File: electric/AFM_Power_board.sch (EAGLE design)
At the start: 16 parts, among them IC1 LM4041CILP, IC2 LM7805_TO220V, IC3 7812T, J2 694103303002

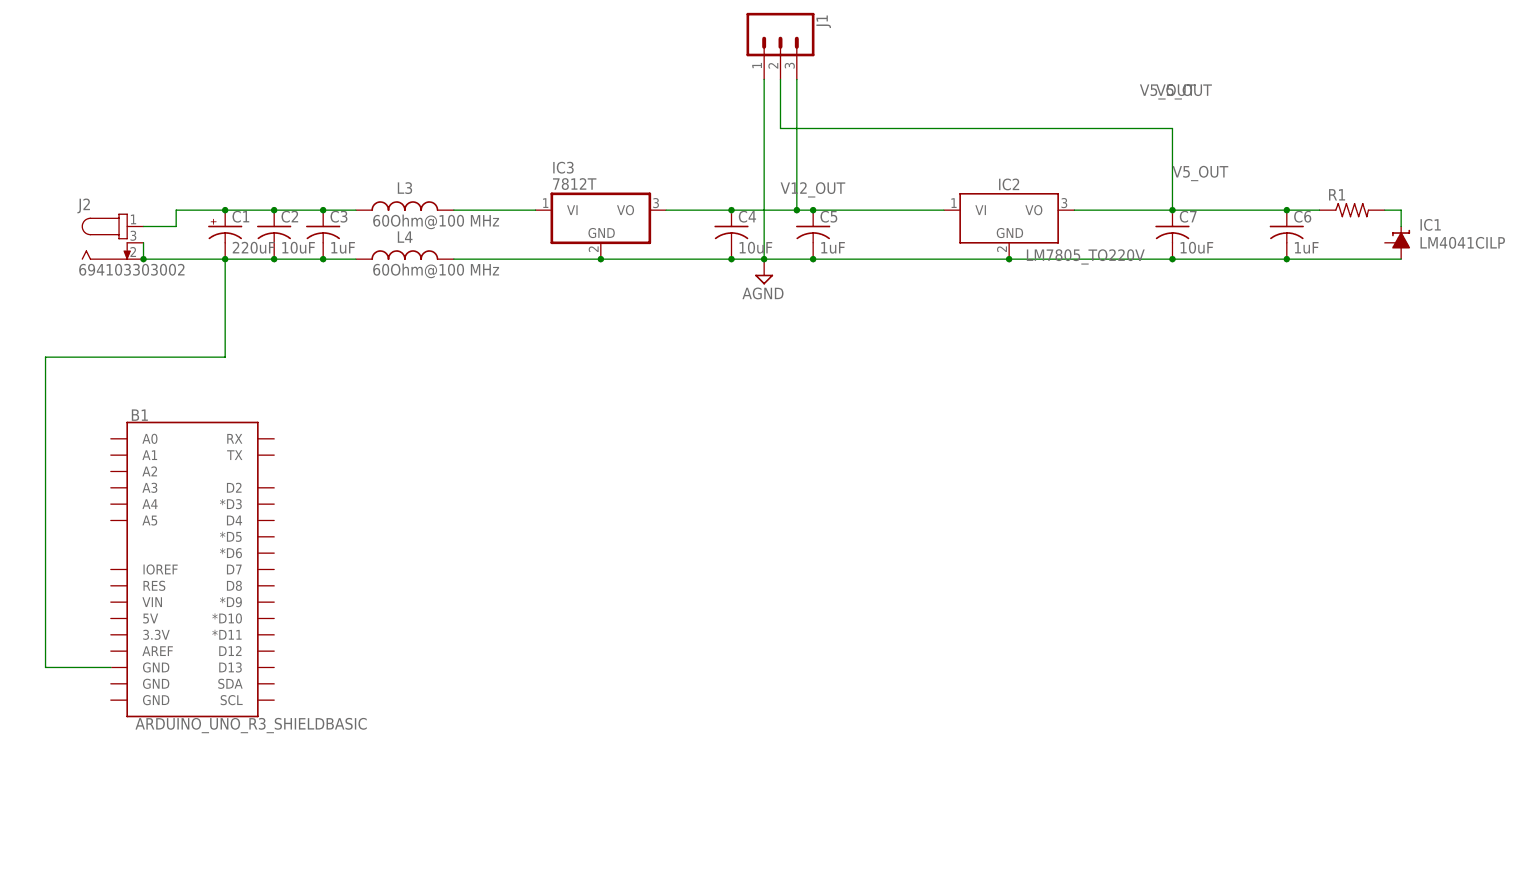
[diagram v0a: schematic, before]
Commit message: allboards
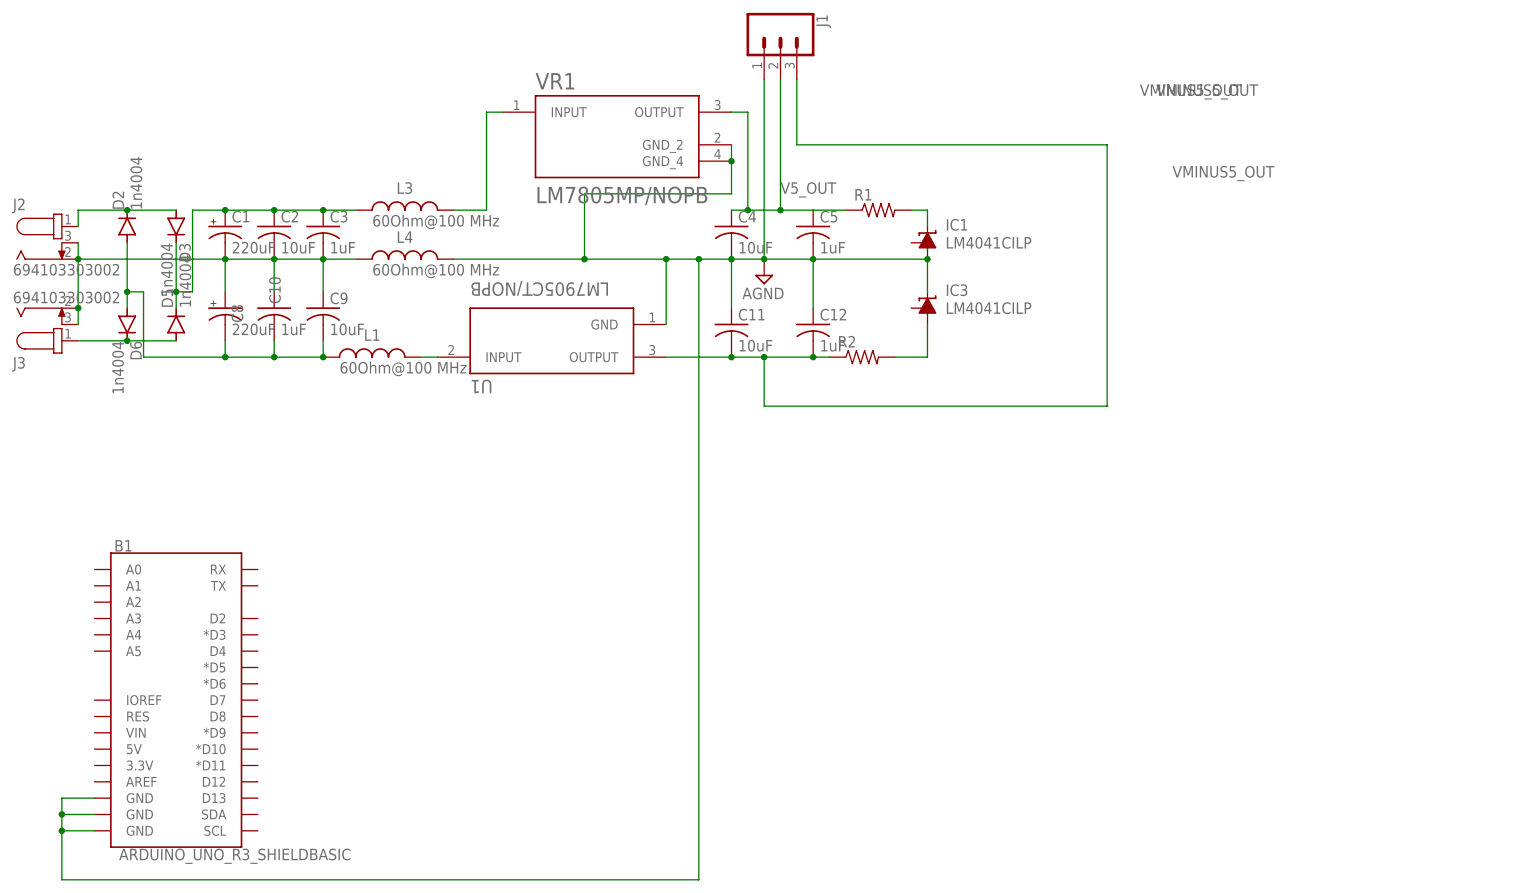
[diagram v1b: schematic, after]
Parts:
- removed C6: 1uF, BeagleBone_Black_Wireless:C-US050-024X044
- removed C7: 10uF, BeagleBone_Black_Wireless:C-US050-024X044
- removed IC2: LM7805_TO220V, IC_Power-Management:LM7805_TO220V
- added C10, C12: 1uF, BeagleBone_Black_Wireless:C-US050-024X044
- added C11, C9: 10uF, BeagleBone_Black_Wireless:C-US050-024X044
- added C8: 220uF, BeagleBone_Blue_R3:CAPACITOR-PE5-8.5
- added D2, D3, D5, D6: 1n4004, diode:DIODE-SOD123
- added J3: 694103303002, DC Power Jacks:694103303002
- added L1: 60Ohm@100 MHz, Wurth_EMC Components_WE-CBF:WE-CBF_0603_74279267_WB_HS
- added R2: (no value), BeagleBone_Black_Wireless:R-US_0204/5
- added U1: LM7905CT/NOPB, LM7905CT_NOPB:LM7905CT/NOPB
- added VR1: LM7805MP/NOPB, LM7805MP_NOPB:LM7805MP/NOPB
- IC3: value 7812T -> LM4041CILP; device adafruit:7812T -> texas:LM4041CILP
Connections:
- removed net N$3: IC3.VI, L3.2
- removed net V12_OUT: C4.1, C5.1, IC2.VI, IC3.VO, J1.3
- new net GROUND: C1.-, C10.1, C2.2, C3.2, C8.+, C9.1, J2.2, J2.3, J3.2, J3.3, L4.1
- new net N$10: C10.2, C8.-, C9.2, D2.A, D6.A, L1.1
- new net N$11: C1.+, C2.1, C3.1, D3.C, D5.C, L3.1
- new net N$8: IC3.A, R2.2
- new net N$9: D5.A, D6.C, J3.1
- new net POWERP: D2.C, D3.A, J2.1
- new net VMINUS5_OUT: C11.2, C12.2, J1.3, R2.1, U1.OUTPUT
- net AGND: now also B1.GND@0, B1.GND@1, B1.GND@2, C11.1, C12.1, IC3.C, U1.GND, VR1.GND_2, VR1.GND_4; no longer C6.2, C7.2, IC2.GND, IC3.GND
- net N$1: now also L3.2, VR1.INPUT; no longer C1.+, C2.1, C3.1, J2.1, L3.1
- net N$2: now also L1.2, U1.INPUT; no longer B1.GND@2, C1.-, C2.2, C3.2, J2.2, J2.3, L4.1
- net V5_OUT: now also C4.1, C5.1, VR1.OUTPUT; no longer C6.1, C7.1, IC2.VO
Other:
- moved on the sheet: B1, IC1, J2, R1
